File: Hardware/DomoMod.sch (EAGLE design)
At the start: 38 parts, among them Q1 BSS138, Q2 BSS138, U1 NCS36000, U2 CCS811, U3 BME280, U4 PIR

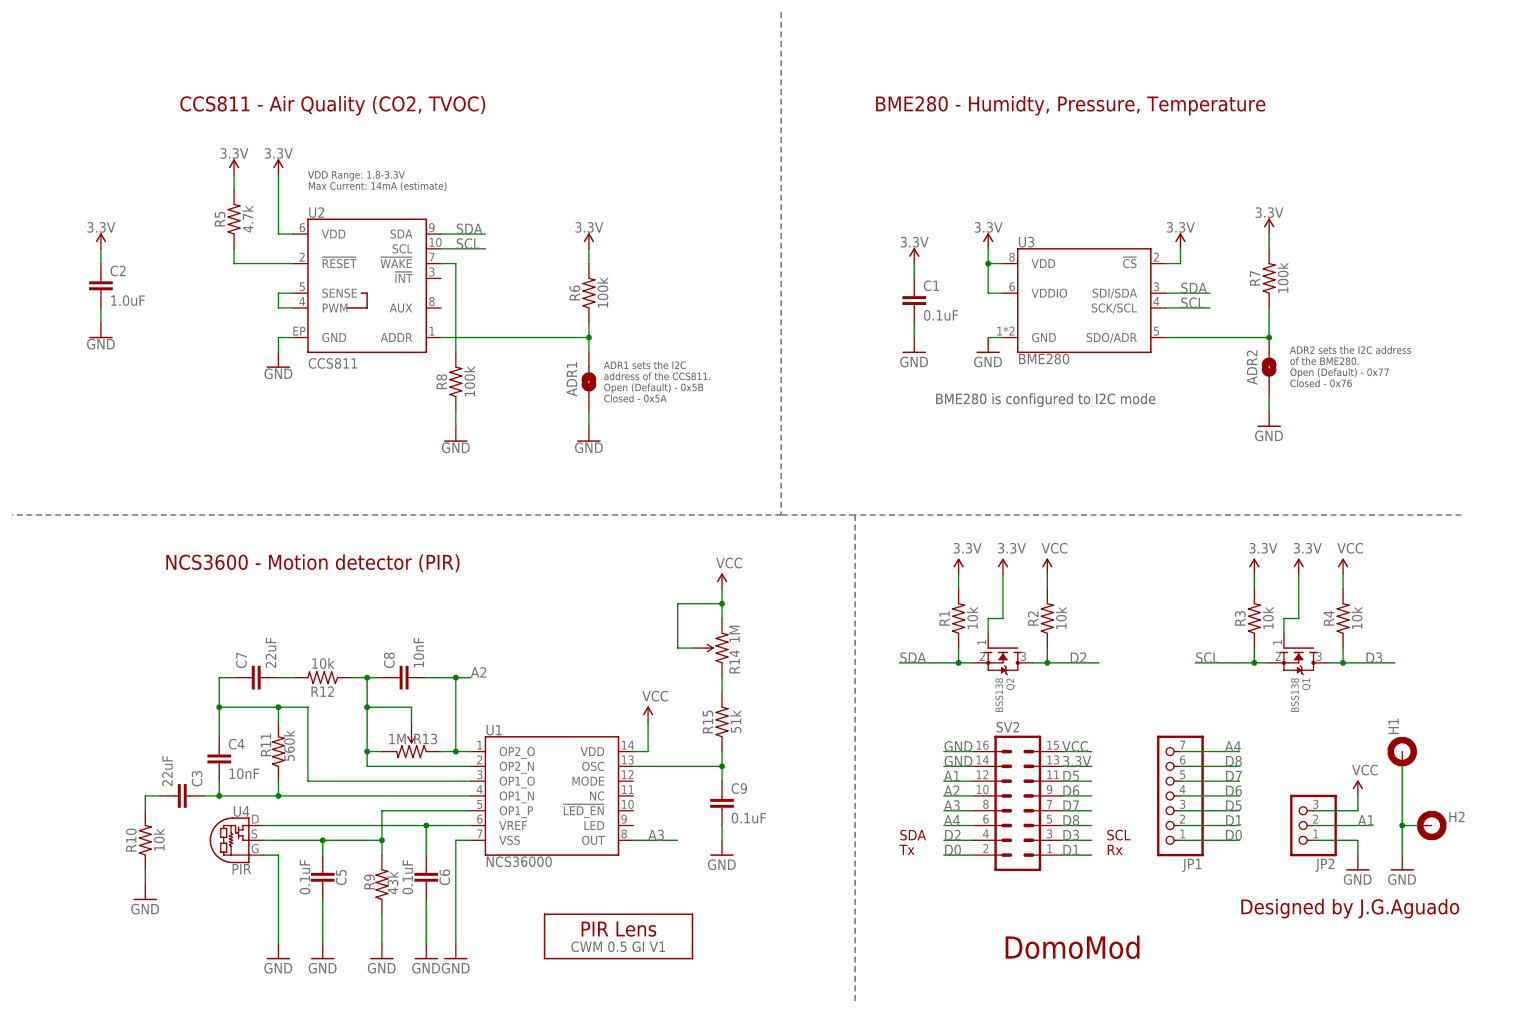
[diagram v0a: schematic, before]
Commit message: Update
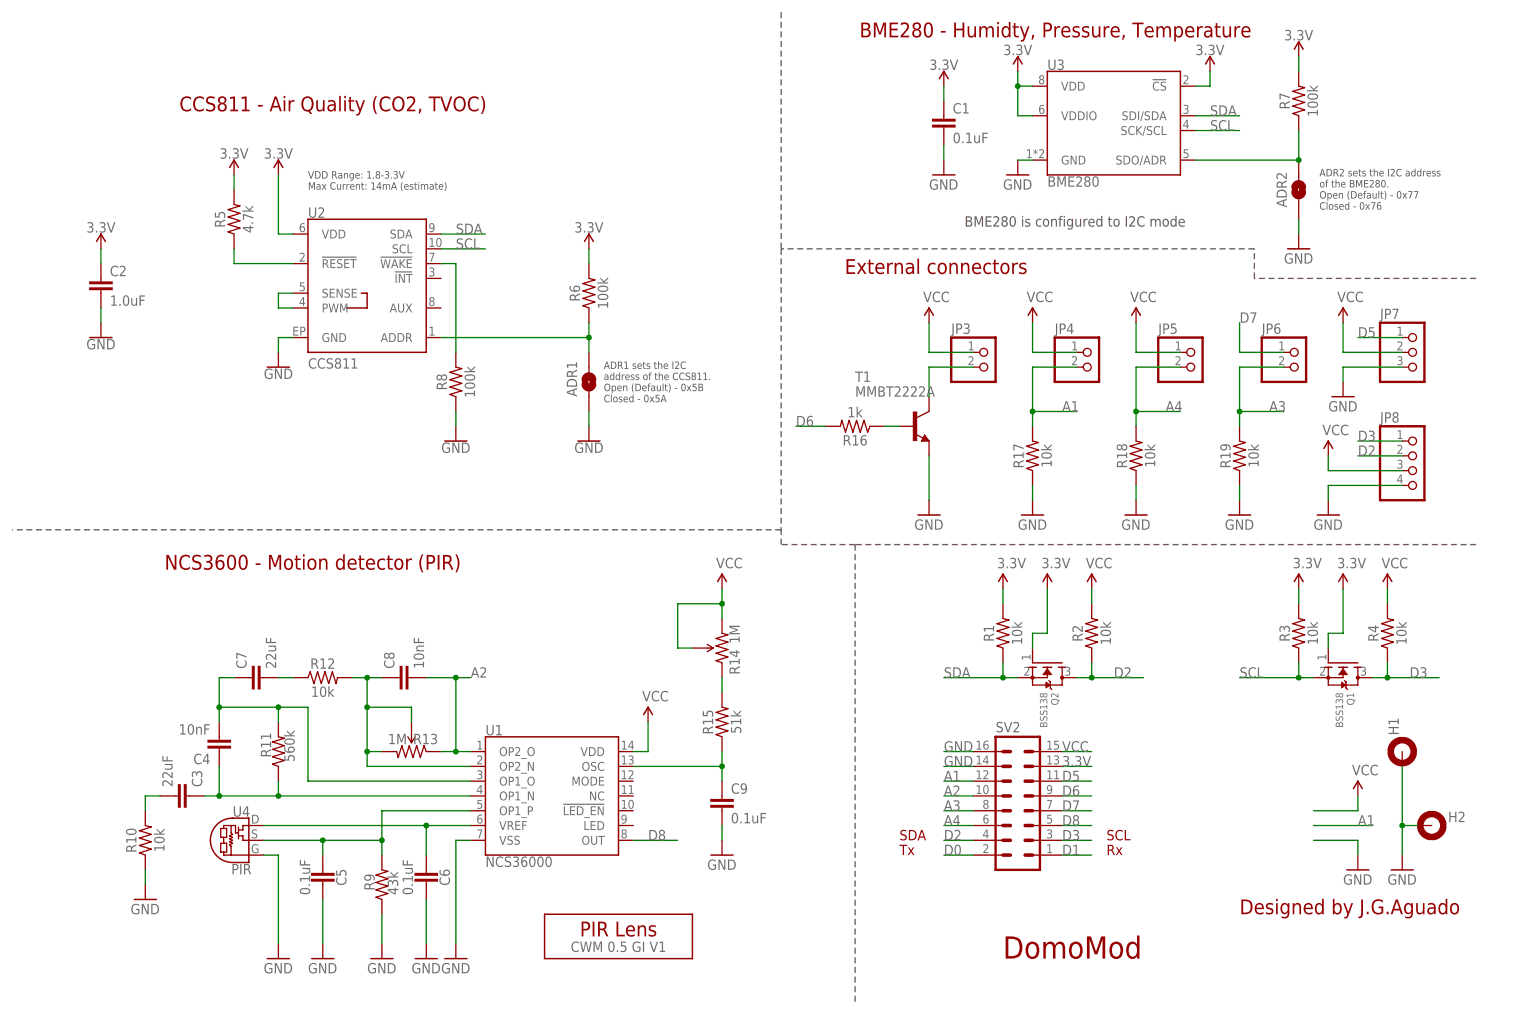
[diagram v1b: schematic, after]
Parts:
- removed JP1: (no value), pinhead:PINHD-1X7/90
- removed JP2: (no value), pinhead:PINHD-1X3
- added JP3, JP4, JP5, JP6: (no value), pinhead:PINHD-1X2
- added JP7: (no value), pinhead:PINHD-1X3
- added JP8: (no value), pinhead:PINHD-1X4
- added R16: 1k, SparkFun-Resistors:100KOHM-0603-1/10W-1%
- added R17, R18, R19: 10k, SparkFun-Resistors:100KOHM-0603-1/10W-1%
- added T1: MMBT2222A, transistor:BC808-NPN-SOT23-BEC
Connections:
- new net N$10: R16.1, T1.B
- new net N$9: JP3.2, T1.C
- net A1: now also JP4.2, R17.2; no longer JP2.2
- net A3: now also JP6.2, R19.2; no longer U1.OUT
- net A4: now also JP5.2, R18.2; no longer JP1.7
- net D0: no longer JP1.1
- net D1: no longer JP1.2
- net D2: now also JP8.2
- net D3: now also JP8.1
- net D5: now also JP7.1; no longer JP1.3
- net D6: now also R16.2; no longer JP1.4
- net D7: now also JP6.1; no longer JP1.5
- net D8: now also U1.OUT; no longer JP1.6
- net GND: now also JP7.3, JP8.4, R17.1, R18.1, R19.1, T1.E; no longer JP2.1
- net N$4: now also R12.1; no longer R12.2
- net N$5: now also C4.1; no longer C4.2
- net N$6: now also C4.2; no longer C4.1
- net N$7: now also R12.2; no longer R12.1
- net VCC: now also JP3.1, JP4.1, JP5.1, JP7.2, JP8.3; no longer JP2.3
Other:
- note added: "External connectors"
- moved on the sheet: ADR2, C1, C4, Q1, Q2, R1, R12, R2, R3, R4, R7, U3
